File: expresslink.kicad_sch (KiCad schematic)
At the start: 10 parts, among them J1 Conn_02x05_Odd_Even, J2 Conn_02x03_Odd_Even, U1 ESP32-C3-MINI-1, Y1 32.768kHz

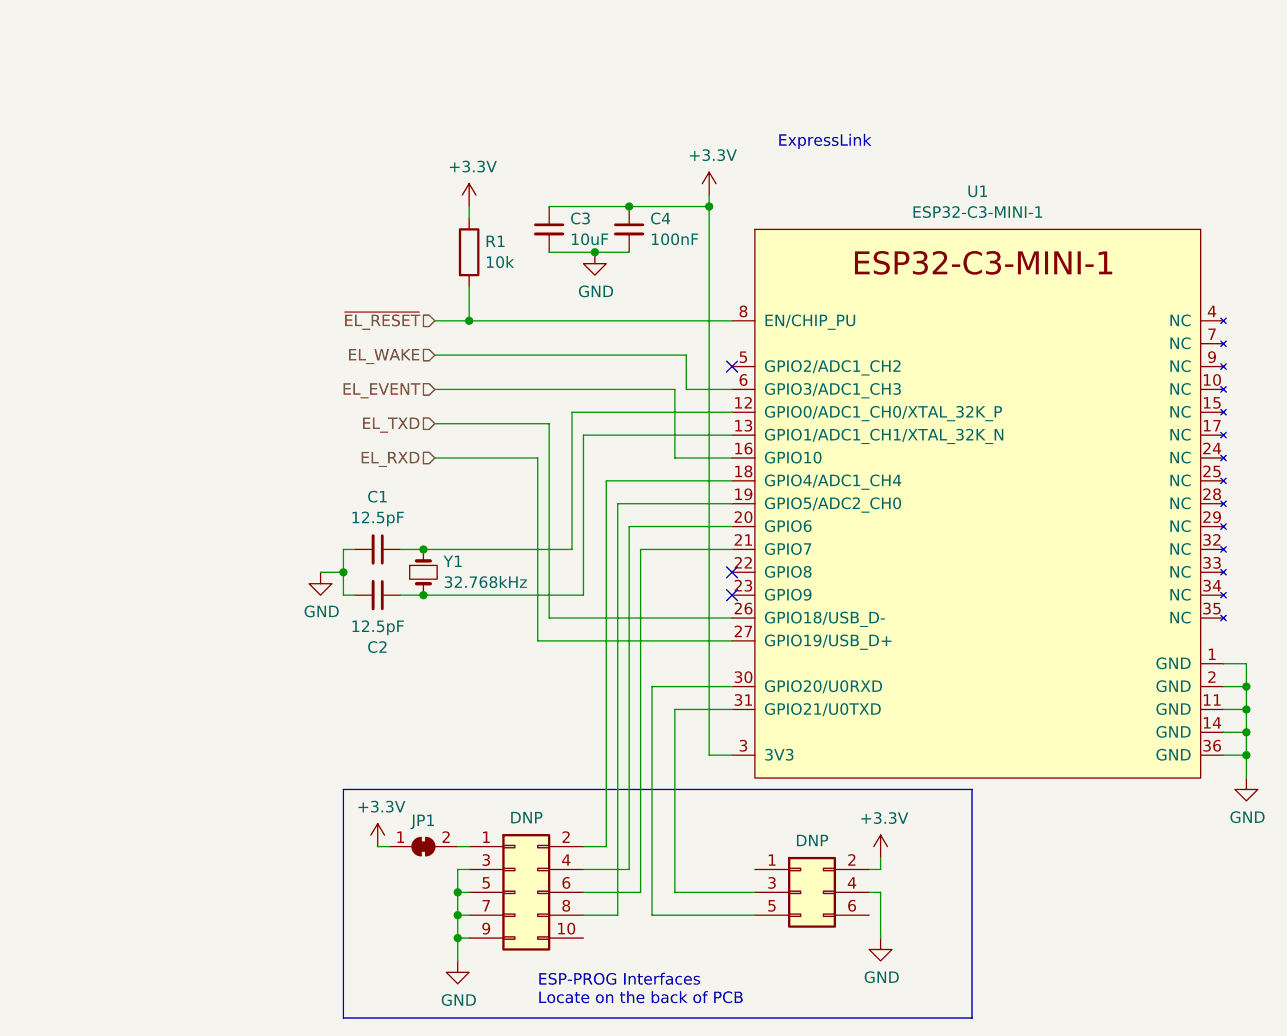
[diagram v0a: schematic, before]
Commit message: updates to the images and place holders for MCU footprint
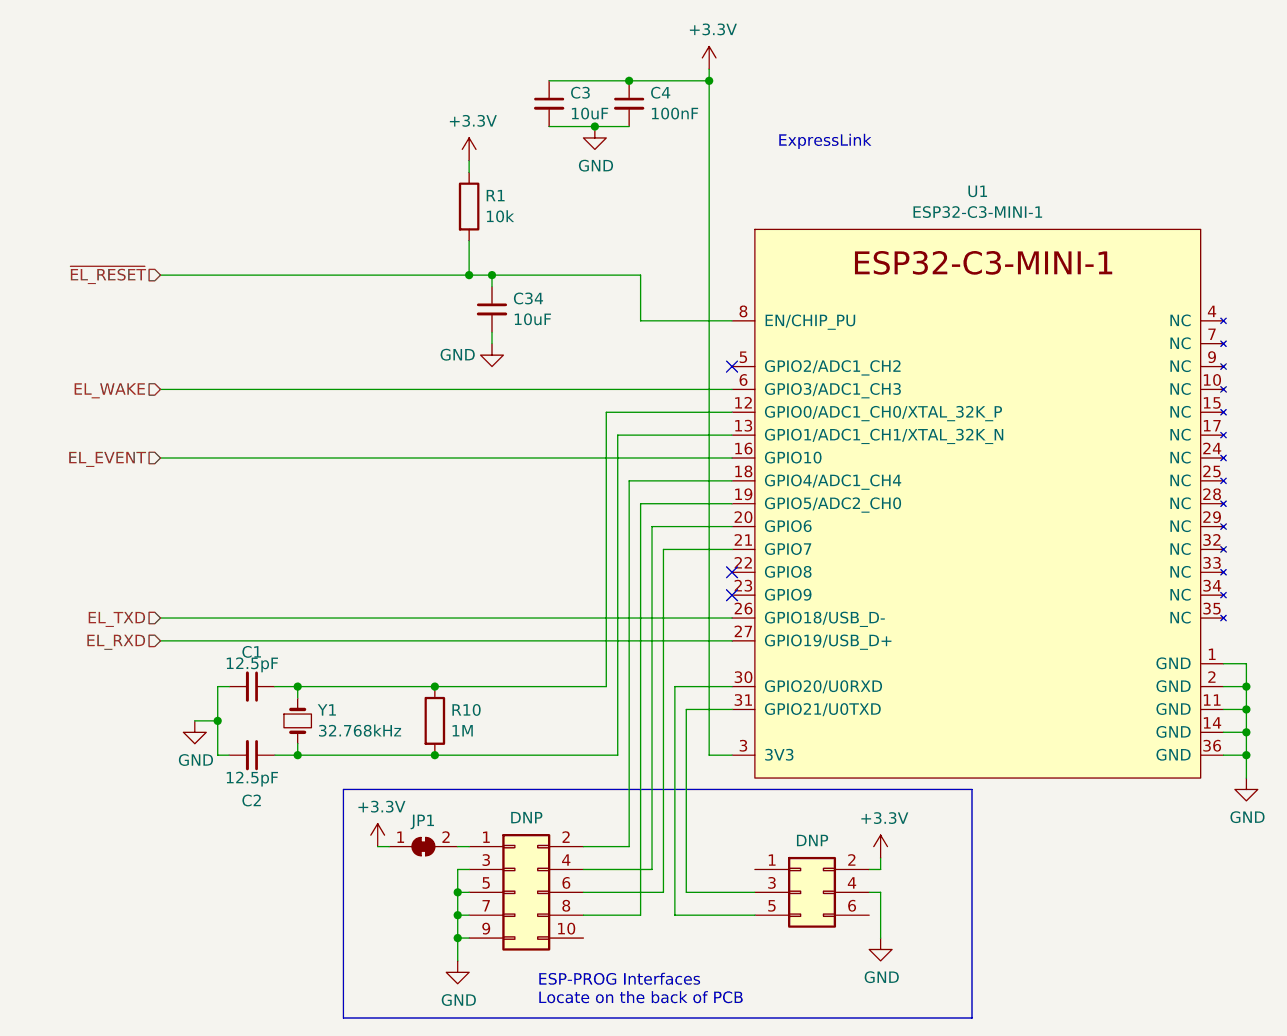
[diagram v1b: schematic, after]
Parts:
- added C34: 10uF, Capacitor_SMD:C_0603_1608Metric_Pad1.08x0.95mm_HandSolder, symbol Device:C_Small
- added R10: 1M, Resistor_SMD:R_0603_1608Metric_Pad0.98x0.95mm_HandSolder, symbol Device:R
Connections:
- net GND: now also C34.2
- net ~{EL_RESET}: now also C34.1
- net at C1.1, U1.12 (GPIO0/ADC1_CH0/XTAL_32K_P), Y1.1: now also R10.1
- net at C2.1, U1.13 (GPIO1/ADC1_CH1/XTAL_32K_N), Y1.2: now also R10.2
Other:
- moved on the sheet: C1, C2, C3, C4, R1, Y1
